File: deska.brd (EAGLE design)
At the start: 68.2 x 54.6 mm, 25 parts, among them Q1 BC547, X1 JST-XH-03-PIN-LONG-PAD, X2 JST-XH-03-PIN-LONG-PAD, X3 JST-XH-03-PIN-LONG-PAD, X4 JST-XH-04-PIN-LONG-PAD, X5 JST-XH-04-PIN-LONG-PAD, X6 JST-XH-04-PIN-LONG-PAD

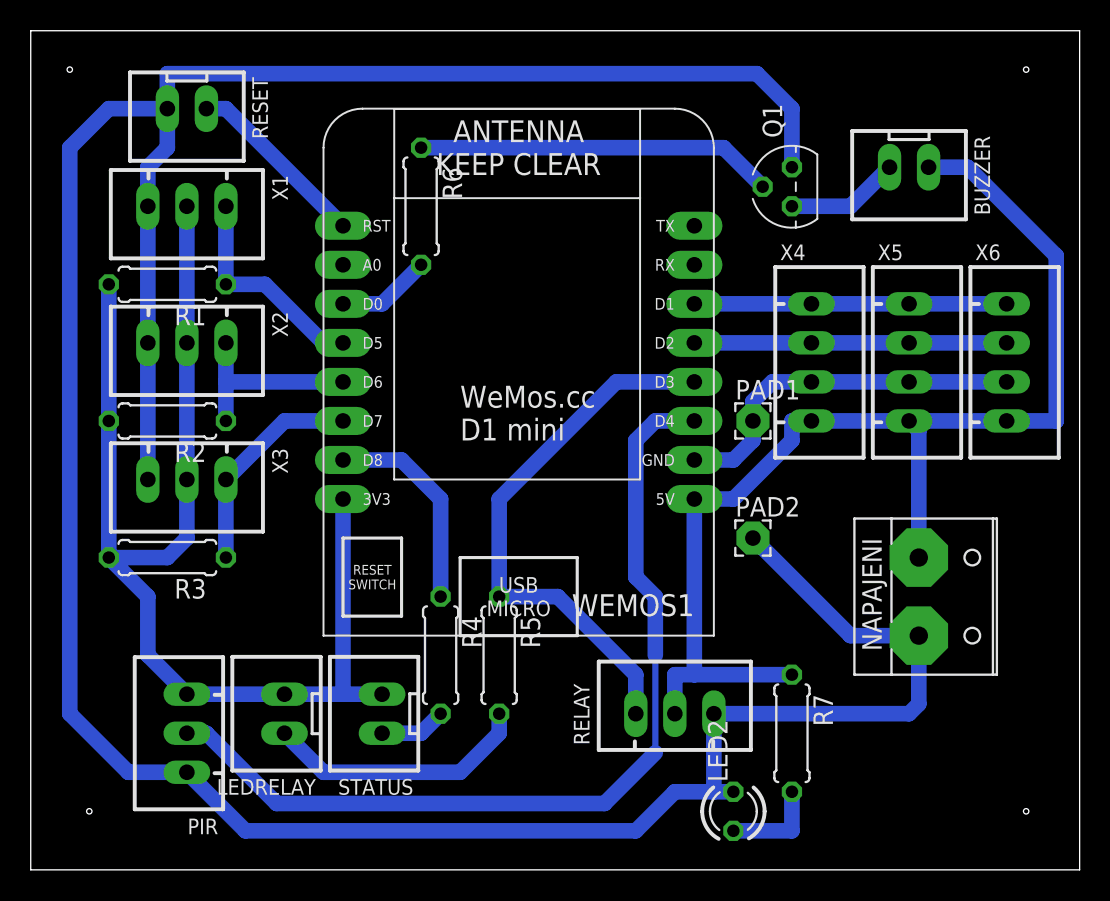
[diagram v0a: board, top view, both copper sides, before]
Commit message: +
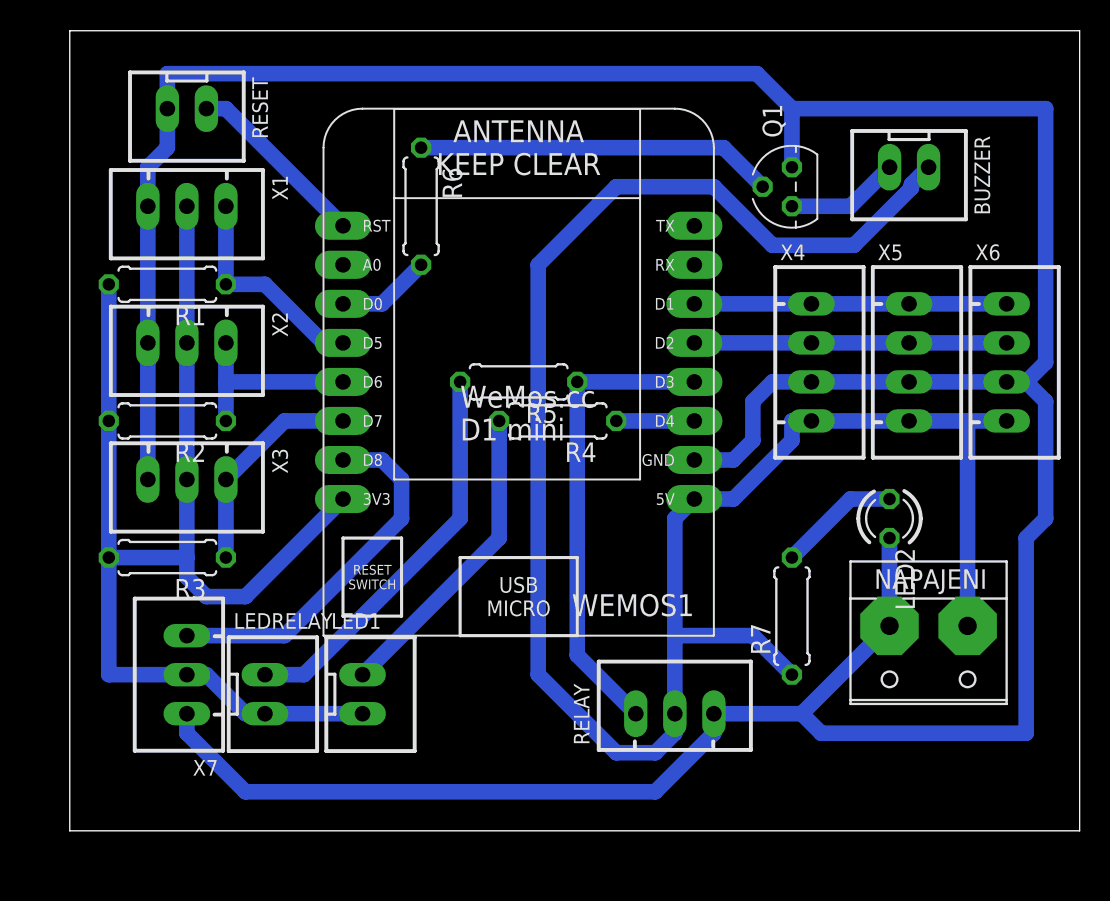
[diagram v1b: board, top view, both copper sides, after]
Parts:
- removed PAD1, PAD2: (no value), wirepad:2,15/1,0
- removed PIR: JST-XH-03-PIN-LONG-PAD, Rembrandt Electronics - JST XH Connectors v1-0:JST-XH-03-PACKAGE-LONG-PAD
- removed STATUS: JST-XH-02-PIN-LONG-PAD, Rembrandt Electronics - JST XH Connectors v1-0:JST-XH-02-PACKAGE-LONG-PAD
- added LED1: JST-XH-02-PIN-LONG-PAD, Rembrandt Electronics - JST XH Connectors v1-0:JST-XH-02-PACKAGE-LONG-PAD
- added X7: JST-XH-03-PIN-LONG-PAD, Rembrandt Electronics - JST XH Connectors v1-0:JST-XH-03-PACKAGE-LONG-PAD
- moved LED2 21.6 mm to (69.8, 25.4), turned to 270 degrees
- moved R5 17.8 mm to (45.7, 34.3), turned to 180 degrees
- moved R4 17.0 mm to (48.3, 31.8), turned to 180 degrees
- moved R7 7.62 mm to (63.5, 19.1), turned to 90 degrees
- moved NAPAJENI 2.54 mm to (72.4, 17.8), turned to 180 degrees
- moved LEDRELAY 1.80 mm to (29.2, 14.0), turned to 270 degrees
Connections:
- net +3V3: now also LED1.2, X7.2; no longer PIR.3, STATUS.2
- net BUILTINLED: now also WEMOS1.D4; no longer WEMOS1.D8
- net GND: now also X7.1; no longer PAD1.1, PAD2.1, PIR.1
- net N$3: now also WEMOS1.D8, X7.3; no longer PIR.2, WEMOS1.D4
- net N$6: now also LED1.1; no longer STATUS.1
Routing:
- net +5V: track 78.6 -> 130.5 mm
- net N$3: track 58.9 -> 24.0 mm
- net N$6: track 4.34 -> 20.2 mm
- net BUILTINLED: track 13.8 -> 5.08 mm
- net N$2: track 17.3 -> 25.8 mm
- net GND: track 224.4 -> 230.9 mm
- net N$14: track 35.7 -> 30.8 mm
- net +3V3: track 81.4 -> 85.5 mm
- net N$4: track 6.35 -> 7.93 mm
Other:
- board size 68.2 x 54.6 mm -> 65.7 x 52.1 mm
